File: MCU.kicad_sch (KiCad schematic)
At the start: 24 parts, among them J8 ICSP_Prog_Header, SW2 Mode, SW3 RST, U8 PIC18F67K22-I/PT, Y1 16MHz

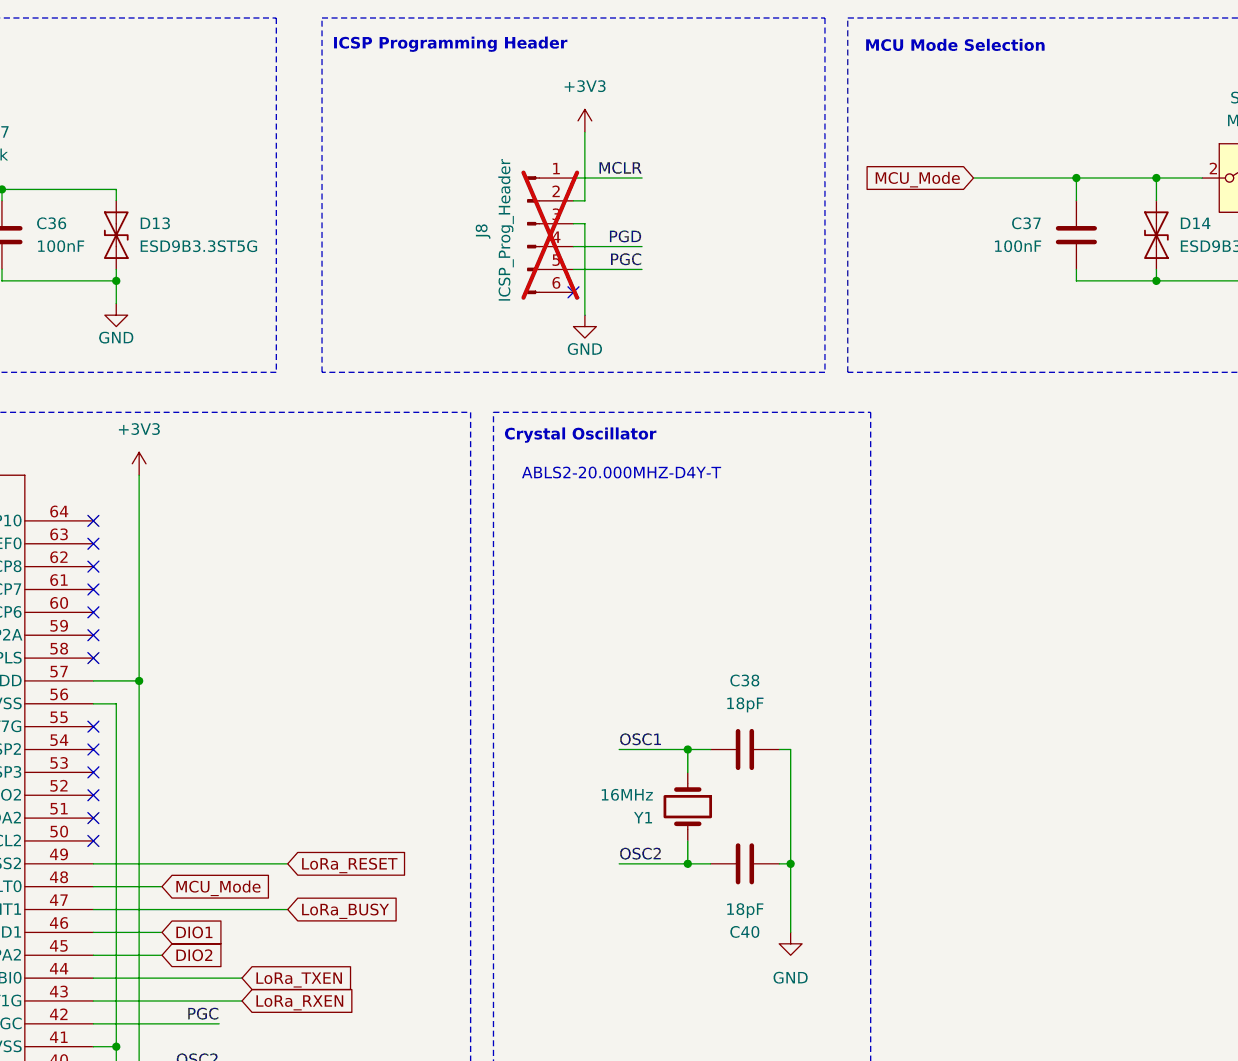
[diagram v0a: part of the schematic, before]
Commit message: reverted back to og files
[local revision r5 4274e03a1d0e]
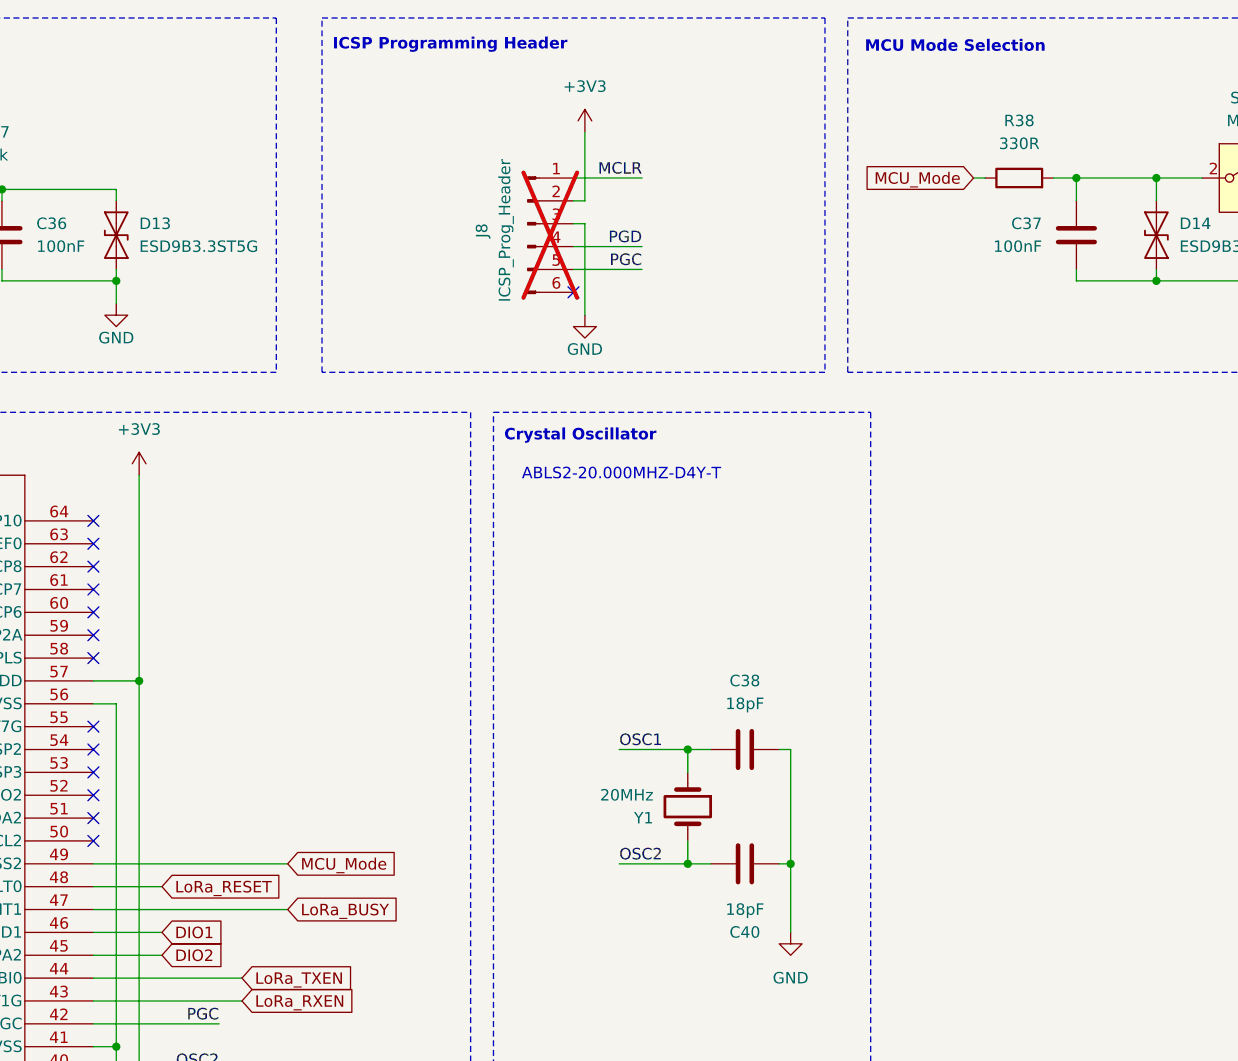
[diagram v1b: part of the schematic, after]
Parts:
- added R38: 330R, Resistor_SMD:R_0805_2012Metric, symbol Device:R
- Y1: value 16MHz -> 20MHz
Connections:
- net LoRa_RESET: now also U8.48 (RB0/INT0/FLT0); no longer U8.49 (RD7/PSP7/*SS2)
- net MCU_Mode: now also U8.49 (RD7/PSP7/*SS2), R38.1; no longer C37.1, D14.2 (A2), SW2.2 (B), U8.48 (RB0/INT0/FLT0)
- new net: C37.1, D14.2 (A2), R38.2, SW2.2 (B)
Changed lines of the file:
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@@
+	(wire
+		(pts
+			(xy 246.38 33.02) (xy 248.92 33.02)
+		)
+		(stroke
+			(width 0)
+			(type default)
+		)
+	)
 	(wire
 		(pts
@@
 	(wire
 		(pts
-			(xy 237.49 33.02) (xy 248.92 33.02)
+			(xy 237.49 33.02) (xy 238.76 33.02)
 		)
 		(stroke
@@
 	(global_label "LoRa_RESET"
 		(shape input)
-		(at 161.29 109.22 0)
+		(at 147.32 111.76 0)
 		(fields_autoplaced yes)
 		(effects
@@
 		)
 		(property "Intersheetrefs" "${INTERSHEET_REFS}"
-			(at 175.584 109.22 0)
+			(at 161.614 111.76 0)
 			(hide yes)
 			(show_name no)
@@
 	(global_label "MCU_Mode"
 		(shape input)
-		(at 147.32 111.76 0)
+		(at 161.29 109.22 0)
 		(fields_autoplaced yes)
 		(effects
@@
 		)
 		(property "Intersheetrefs" "${INTERSHEET_REFS}"
-			(at 160.1627 111.76 0)
+			(at 174.1327 109.22 0)
 			(hide yes)
 			(show_name no)
@@
 	)
 	(symbol
+		(lib_id "Device:R")
+		(at 242.57 33.02 90)
+		(unit 1)
+		(body_style 1)
+		(exclude_from_sim no)
+		(in_bom yes)
+		(on_board yes)
+		(in_pos_files yes)
+		(dnp no)
+		(fields_autoplaced yes)
+		(property "Reference" "R38"
+			(at 242.57 26.67 90)
+			(show_name no)
+			(do_not_autoplace no)
+			(effects
+				(font
+					(size 1.27 1.27)
+				)
+			)
+		)
+		(property "Value" "330R"
+			(at 242.57 29.21 90)
+			(show_name no)
+			(do_not_autoplace no)
+			(effects
+				(font
+					(size 1.27 1.27)
+				)
+			)
+		)
+		(property "Footprint" "Resistor_SMD:R_0805_2012Metric"
+			(at 242.57 34.798 90)
+			(hide yes)
+			(show_name no)
+			(do_not_autoplace no)
+			(effects
+				(font
+					(size 1.27 1.27)
+				)
+			)
+		)
+		(property "Datasheet" ""
+			(at 242.57 33.02 0)
+			(hide yes)
+			(show_name no)
+			(do_not_autoplace no)
+			(effects
+				(font
+					(size 1.27 1.27)
+				)
+			)
+		)
+		(property "Description" "Resistor"
+			(at 242.57 33.02 0)
+			(hide yes)
+			(show_name no)
+			(do_not_autoplace no)
+			(effects
+				(font
+					(size 1.27 1.27)
+				)
+			)
+		)
+		(pin "1"
+		)
+		(pin "2"
+		)
+		(instances
+			(project "Demo Project"
+				(path "/4e55511c-c365-4512-9b57-837a9ec6e386/9d40519f-9a51-4d6f-ac34-7f912ff4c2a7"
+					(reference "R38")
+					(unit 1)
+				)
+			)
+		)
+	)
+	(symbol
 		(lib_id "Connector:TestPoint")
 		(at 48.26 41.91 180)
@@
 			)
 		)
-		(property "Value" "16MHz"
+		(property "Value" "20MHz"
 			(at 201.93 101.6001 90)
 			(show_name no)

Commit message: testing plugin
[local revision r3 cb60daacd4a3]
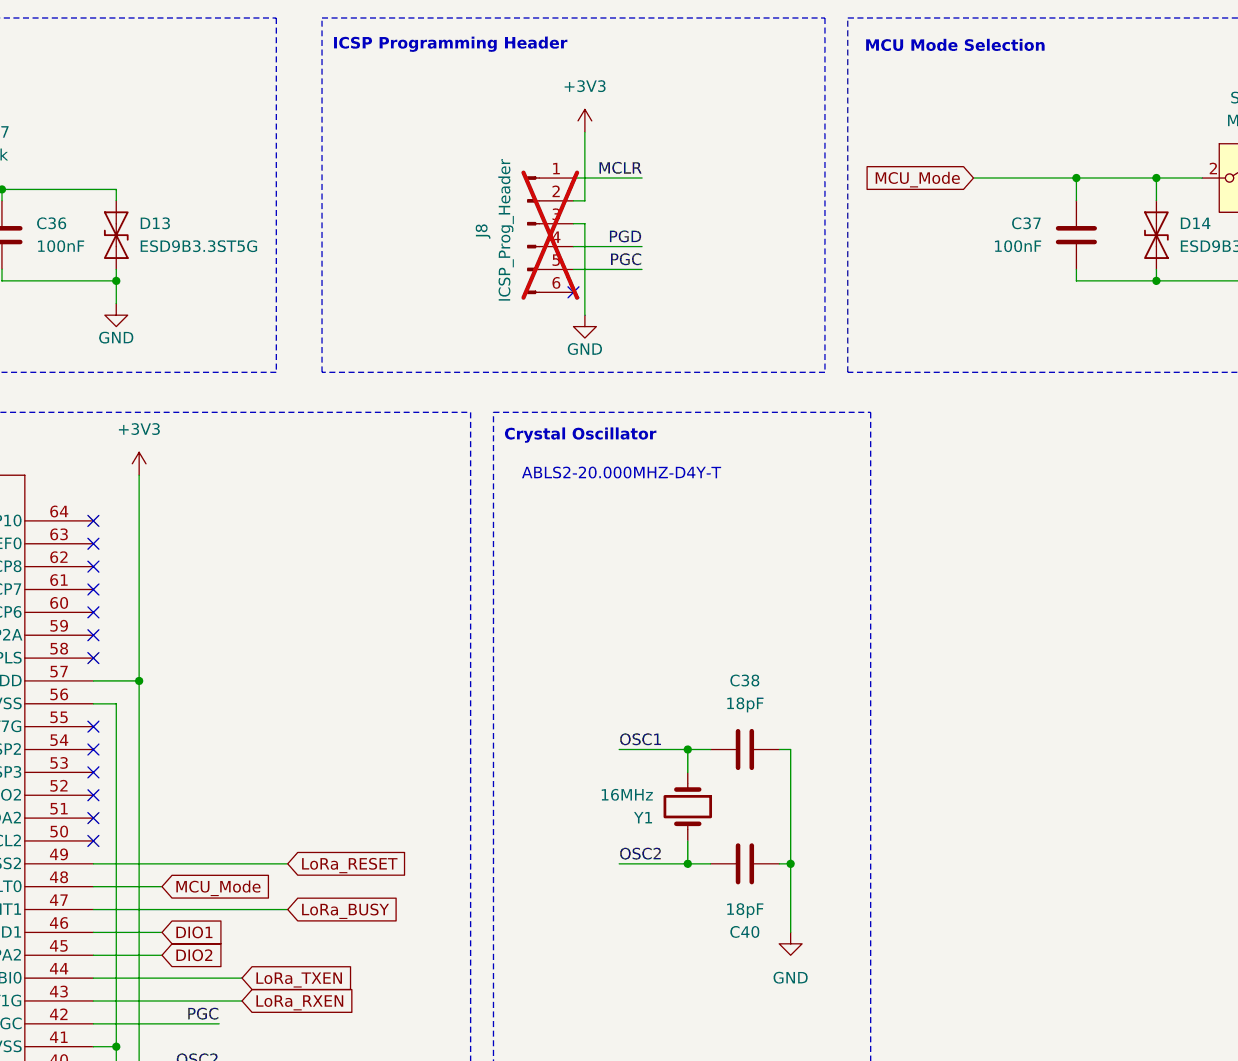
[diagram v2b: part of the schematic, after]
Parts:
- removed R38: 330R, Resistor_SMD:R_0805_2012Metric, symbol Device:R
- Y1: value 20MHz -> 16MHz
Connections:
- net LoRa_RESET: now also U8.49 (RD7/PSP7/*SS2); no longer U8.48 (RB0/INT0/FLT0)
- net MCU_Mode: now also C37.1, D14.2 (A2), SW2.2 (B), U8.48 (RB0/INT0/FLT0); no longer U8.49 (RD7/PSP7/*SS2)
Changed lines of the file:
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@@
-	(wire
-		(pts
-			(xy 246.38 33.02) (xy 248.92 33.02)
-		)
-		(stroke
-			(width 0)
-			(type default)
-		)
-	)
 	(wire
 		(pts
@@
 	(wire
 		(pts
-			(xy 237.49 33.02) (xy 238.76 33.02)
+			(xy 237.49 33.02) (xy 248.92 33.02)
 		)
 		(stroke
@@
 	(global_label "LoRa_RESET"
 		(shape input)
-		(at 147.32 111.76 0)
+		(at 161.29 109.22 0)
 		(fields_autoplaced yes)
 		(effects
@@
 		)
 		(property "Intersheetrefs" "${INTERSHEET_REFS}"
-			(at 161.614 111.76 0)
+			(at 175.584 109.22 0)
 			(hide yes)
 			(show_name no)
@@
 	(global_label "MCU_Mode"
 		(shape input)
-		(at 161.29 109.22 0)
+		(at 147.32 111.76 0)
 		(fields_autoplaced yes)
 		(effects
@@
 		)
 		(property "Intersheetrefs" "${INTERSHEET_REFS}"
-			(at 174.1327 109.22 0)
+			(at 160.1627 111.76 0)
 			(hide yes)
 			(show_name no)
@@
 	)
 	(symbol
-		(lib_id "Device:R")
-		(at 242.57 33.02 90)
-		(unit 1)
-		(body_style 1)
-		(exclude_from_sim no)
-		(in_bom yes)
-		(on_board yes)
-		(in_pos_files yes)
-		(dnp no)
-		(fields_autoplaced yes)
-		(property "Reference" "R38"
-			(at 242.57 26.67 90)
-			(show_name no)
-			(do_not_autoplace no)
-			(effects
-				(font
-					(size 1.27 1.27)
-				)
-			)
-		)
-		(property "Value" "330R"
-			(at 242.57 29.21 90)
-			(show_name no)
-			(do_not_autoplace no)
-			(effects
-				(font
-					(size 1.27 1.27)
-				)
-			)
-		)
-		(property "Footprint" "Resistor_SMD:R_0805_2012Metric"
-			(at 242.57 34.798 90)
-			(hide yes)
-			(show_name no)
-			(do_not_autoplace no)
-			(effects
-				(font
-					(size 1.27 1.27)
-				)
-			)
-		)
-		(property "Datasheet" ""
-			(at 242.57 33.02 0)
-			(hide yes)
-			(show_name no)
-			(do_not_autoplace no)
-			(effects
-				(font
-					(size 1.27 1.27)
-				)
-			)
-		)
-		(property "Description" "Resistor"
-			(at 242.57 33.02 0)
-			(hide yes)
-			(show_name no)
-			(do_not_autoplace no)
-			(effects
-				(font
-					(size 1.27 1.27)
-				)
-			)
-		)
-		(pin "1"
-		)
-		(pin "2"
-		)
-		(instances
-			(project "Demo Project"
-				(path "/4e55511c-c365-4512-9b57-837a9ec6e386/9d40519f-9a51-4d6f-ac34-7f912ff4c2a7"
-					(reference "R38")
-					(unit 1)
-				)
-			)
-		)
-	)
-	(symbol
 		(lib_id "Connector:TestPoint")
 		(at 48.26 41.91 180)
@@
 			)
 		)
-		(property "Value" "20MHz"
+		(property "Value" "16MHz"
 			(at 201.93 101.6001 90)
 			(show_name no)
